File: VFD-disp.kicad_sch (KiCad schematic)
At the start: 96 parts, among them J1 USB_C_Receptacle_USB2.0_14P, J10 Conn_02x03_Odd_Even, J11 Conn_02x03_Odd_Even, J2 Conn_01x04_MountingPin, J3 Jack-DC, J8 Conn_02x03_Odd_Even, J9 Conn_02x03_Odd_Even, Q1 NMOS, Q3 NMOS, SW1 SW_SPST, U1 ESP32-C6-WROOM-1, U11 MAX811TEUS-T, U12 MCP4728, U2 FUSB302B01MPX, U3 LM1117DT-3.3, U4 MCP1416, U5 LM2576HVS-ADJ, U6 MAX1771xSA, U7 LM2576HVS-ADJ, U8 L7812, U9 FM24C64B, Y1 Crystal

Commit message: Make schematic ready for routing
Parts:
- removed F2: Fuse, Fuse:Fuse_0805_2012Metric, symbol Device:Fuse
- removed J10, J8: Conn_02x03_Odd_Even, Connector_PinSocket_2.54mm:PinSocket_2x03_P2.54mm_Horizontal, symbol Connector_Generic:Conn_02x03_Odd_Even
- removed J11, J9: Conn_02x03_Odd_Even, Connector_PinHeader_2.54mm:PinHeader_2x03_P2.54mm_Horizontal, symbol Connector_Generic:Conn_02x03_Odd_Even
- removed J2: Conn_01x04_MountingPin, Connector_JST:JST_SH_BM04B-SRSS-TB_1x04-1MP_P1.00mm_Vertical, symbol Connector_Generic_MountingPin:Conn_01x04_MountingPin
- removed R23: R, Resistor_SMD:R_0805_2012Metric, symbol Device:R
- added C19, C30, C31, C32, C33, C35: C, Capacitor_SMD:C_0805_2012Metric, symbol Device:C
- added C34: C_Polarized, Capacitor_Tantalum_SMD:CP_EIA-7343-31_Kemet-D, symbol Device:C_Polarized
- added J2, J5: Conn_02x04_Odd_Even, Connector_PinSocket_2.54mm:PinSocket_2x04_P2.54mm_Horizontal, symbol Connector_Generic:Conn_02x04_Odd_Even
- added J4, J6: Conn_02x04_Odd_Even, Connector_PinHeader_2.54mm:PinHeader_2x04_P2.54mm_Horizontal, symbol Connector_Generic:Conn_02x04_Odd_Even
- added R21: R, Resistor_SMD:R_0805_2012Metric, symbol Device:R
- added U10: TXS0104EPW, Package_SO:TSSOP-14_4.4x5mm_P0.65mm, symbol Logic_LevelTranslator:TXS0104EPW
- C18: footprint (none) -> Capacitor_SMD:C_0805_2012Metric
- R7: footprint (none) -> Resistor_SMD:R_0805_2012Metric
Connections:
- net +12V: no longer R3.1, U6.2 (V+)
- net +3.3V: now also R22.1, R3.1, C30.1, R21.1, U10.1 (V_{CCA})
- net +5V: now also C19.1, C33.1, C34.1, U10.14 (V_{CCB})
- net BLANKING: now also U10.11 (B3); no longer U1.17 (GPIO19)
- net CLOCK: now also U10.12 (B2); no longer U1.16 (GPIO18)
- net DATA_IN: now also U10.13 (B1); no longer U1.23 (GPIO15)
- net F_EN: now also R17.1, U1.19 (GPIO21); no longer R17.2
- net F_PWM: no longer U1.19 (GPIO21)
- net GND: now also R17.2, C19.2, C30.2, C31.2, C32.2, C33.2, C34.2, C35.2, J2.5 (Pin_5), J2.6 (Pin_6), J2.7 (Pin_7), J2.8 (Pin_8), J4.5 (Pin_5), J4.6 (Pin_6), J4.7 (Pin_7), J4.8 (Pin_8), J5.3 (Pin_3), J5.5 (Pin_5), J5.6 (Pin_6), J5.7 (Pin_7), J5.8 (Pin_8), J6.3 (Pin_3), J6.5 (Pin_5), J6.6 (Pin_6), J6.7 (Pin_7), J6.8 (Pin_8), U10.7 (GND), U10.8 (OE)
- net STROBE: now also U10.10 (B4); no longer U1.18 (GPIO20)
- net VBUS: now also U6.2 (V+), C35.1, J2.1 (Pin_1), J2.2 (Pin_2), J2.3 (Pin_3), J2.4 (Pin_4), J4.1 (Pin_1), J4.2 (Pin_2), J4.3 (Pin_3), J4.4 (Pin_4); no longer R17.1
- net TX2: now reaches U1.20 (GPIO22)
- net TX2: now also J6.4 (Pin_4)
- net RX2: now reaches U1.21 (GPIO23)
- net RX2: now also J6.2 (Pin_2)
- net at U1.26 (GPIO3/ADC1_CH3): now also R19.2, R20.1
- net at U1.27 (GPIO2/ADC1_CH2): now also C18.1, R15.2, R18.1
- net at J1.B5 (CC2), U2.1 (CC2), U2.14 (CC2): now also C32.1
- net at J1.A5 (CC1), U2.10 (CC1), U2.11 (CC1): now also C31.1
- net DATA_OUT: no longer names the net of HV5812WG2.2 (DATAOUT)
- net HV_EN renamed /HV_EN
- net RX renamed RX1
- net RX1: now also J5.4 (Pin_4)
- net TX renamed FORWARD_DETECT
- net FORWARD_DETECT: now also U1.5 (MTDI/GPIO5/ADC1_CH5), J6.1 (Pin_1); no longer U1.25 (U0TXD/GPIO16)
- new net: U1.23 (GPIO15), U10.2 (A1)
- new net: U1.16 (GPIO18), U10.3 (A2)
- new net: U1.17 (GPIO19), U10.4 (A3)
- new net: U1.18 (GPIO20), U10.5 (A4)
- new net BACKWARD_DETECT: J5.1 (Pin_1), R21.2, U1.4 (MTMS/GPIO4/ADC1_CH4)
- new net TX1: J5.2 (Pin_2), U1.25 (U0TXD/GPIO16)
- no-connect marks 15 -> 16
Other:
- moved on the sheet: C15, C16, C17, C18, C27, C29, R13, R14, R15, R17, R18, R19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

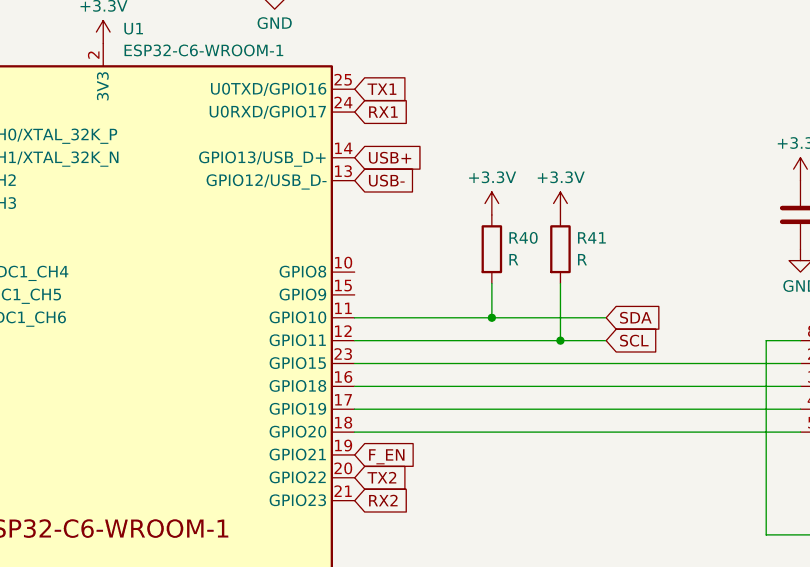
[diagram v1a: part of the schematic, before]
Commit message: WIP płytka
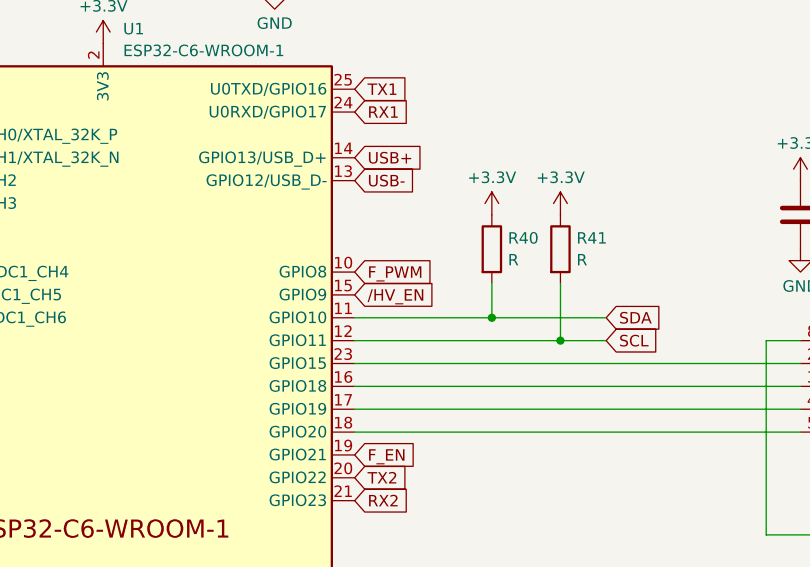
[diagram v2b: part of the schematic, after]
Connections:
- net F_PWM: now also U1.10 (GPIO8)
- net /HV_EN: now also U1.15 (GPIO9)
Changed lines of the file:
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@@
+		)
+	)
+	(global_label "F_PWM"
+		(shape input)
+		(at 224.79 102.87 0)
+		(fields_autoplaced yes)
+		(effects
+			(font
+				(size 1.27 1.27)
+			)
+			(justify left)
+		)
+		(property "Intersheetrefs" "${INTERSHEET_REFS}"
+			(at 234.0042 102.87 0)
+			(effects
+				(font
+					(size 1.27 1.27)
+				)
+				(justify left)
+				(hide yes)
+			)
 		)
 	)
@@
 				(hide yes)
 			)
+		)
+	)
+	(global_label "{slash}HV_EN"
+		(shape input)
+		(at 224.79 105.41 0)
+		(fields_autoplaced yes)
+		(effects
+			(font
+				(size 1.27 1.27)
+			)
+			(justify left)
+		)
+		(property "Intersheetrefs" "${INTERSHEET_REFS}"
+			(at 234.9719 105.41 0)
+			(effects
+				(font
+					(size 1.27 1.27)
+				)
+				(justify left)
+				(hide yes)
+			)

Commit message: WIP płytka
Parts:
- removed C10, C9: C_Polarized, Capacitor_SMD:CP_Elec_5x4.5, symbol Device:C_Polarized
- removed C14, C8: C, Capacitor_SMD:C_0805_2012Metric, symbol Device:C
- removed U8: L7812, Package_TO_SOT_SMD:TO-252-2, symbol Regulator_Linear:L7812
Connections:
- net USB+ is gone; now on net USB_D+: U1.14 (GPIO13/USB_D+)
- net USB- is gone; now on net USB_D-: U1.13 (GPIO12/USB_D-)
- net BACKWARD_DETECT: now also U1.5 (MTDI/GPIO5/ADC1_CH5); no longer U1.4 (MTMS/GPIO4/ADC1_CH4)
- net FORWARD_DETECT: now also J6.3 (Pin_3), U1.4 (MTMS/GPIO4/ADC1_CH4); no longer J6.1 (Pin_1), U1.5 (MTDI/GPIO5/ADC1_CH5)
- net GND: now also J5.2 (Pin_2), J5.4 (Pin_4), J6.1 (Pin_1), J6.2 (Pin_2), J6.4 (Pin_4); no longer J5.5 (Pin_5), J5.7 (Pin_7), J6.3 (Pin_3), J6.5 (Pin_5), J6.7 (Pin_7)
- net RX1: now also J6.5 (Pin_5); no longer J5.4 (Pin_4)
- net RX2: now also J5.7 (Pin_7); no longer J6.2 (Pin_2)
- net TX1: now also J6.7 (Pin_7); no longer J5.2 (Pin_2)
- net TX2: now also J5.5 (Pin_5); no longer J6.4 (Pin_4)
- net at R4.1, U6.8 (CS): now also Q1.1 (D); no longer Q1.3 (S)
- net at D1.2 (A), L1.2: now also Q1.3 (S); no longer Q1.1 (D)
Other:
- moved on the sheet: R22

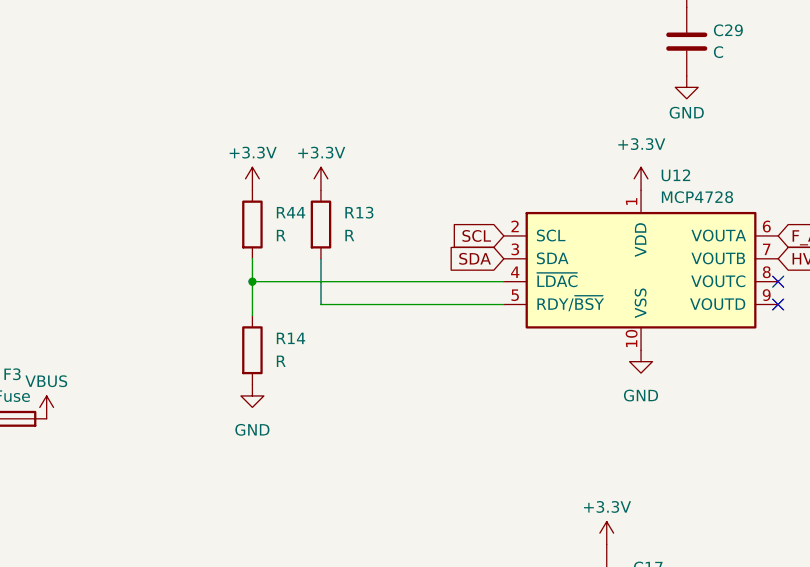
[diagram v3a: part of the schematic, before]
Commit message: WIP płytka
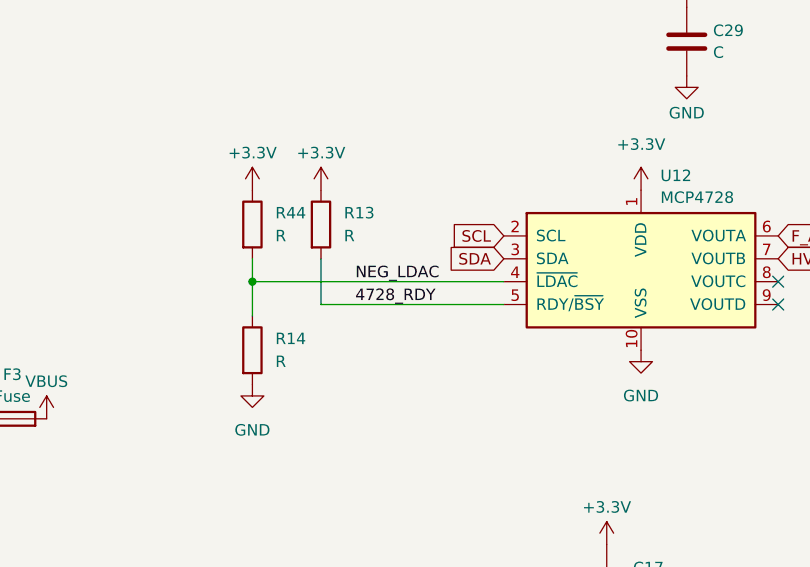
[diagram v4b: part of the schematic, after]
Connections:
- net 4728_RDY: now reaches R13.2, U12.5 (RDY/~{BSY})
- net NEG_LDAC: now reaches R14.1, R44.2, U12.4 (~{LDAC})
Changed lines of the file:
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@@
+		)
+	)
+	(label "4728_RDY"
+		(at 87.63 304.8 0)
+		(effects
+			(font
+				(size 1.27 1.27)
+			)
+			(justify left bottom)
 		)
 	)
@@
 		(effects
 			(font
+				(size 1.27 1.27)
+			)
+			(justify left bottom)
+		)
+	)
+	(label "NEG_LDAC"
+		(at 87.63 302.26 0)
+		(effects
+			(font

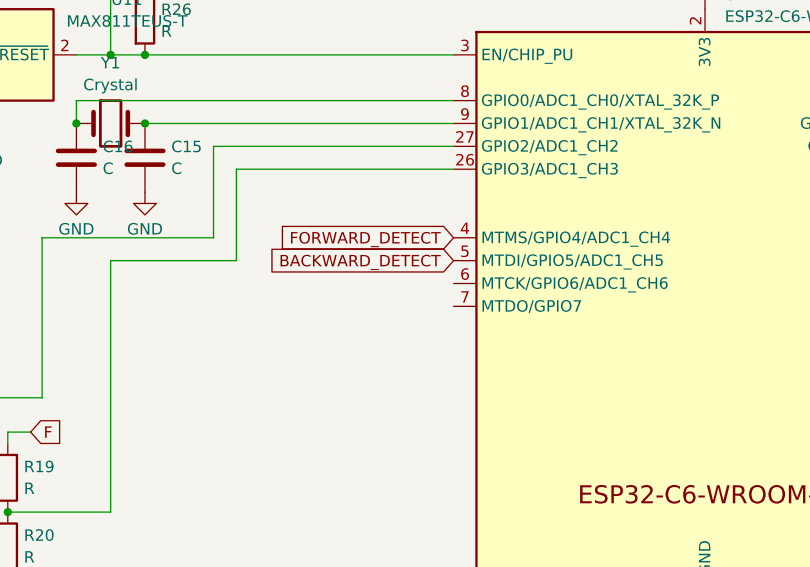
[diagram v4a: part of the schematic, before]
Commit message: WIP płytka
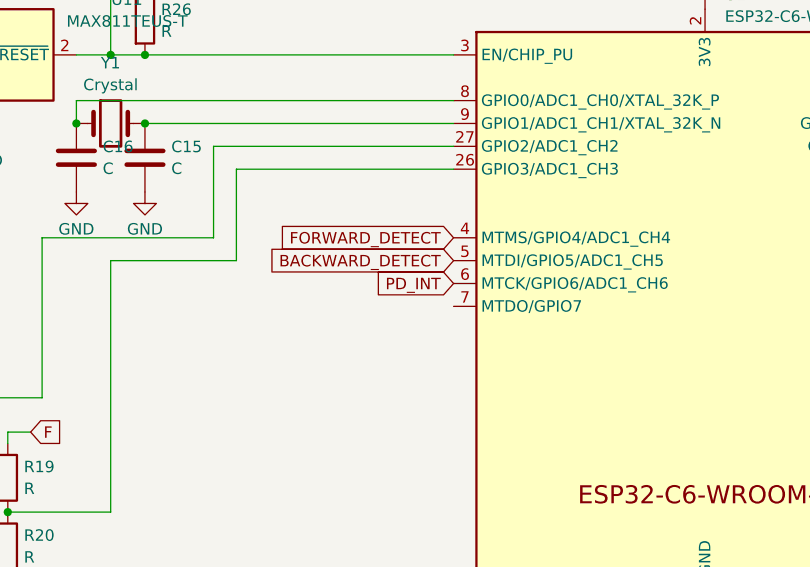
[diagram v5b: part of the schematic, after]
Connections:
- net PD_INT: now also U1.6 (MTCK/GPIO6/ADC1_CH6)
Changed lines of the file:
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@@
+		)
+	)
+	(global_label "PD_INT"
+		(shape input)
+		(at 168.91 107.95 180)
+		(fields_autoplaced yes)
+		(effects
+			(font
+				(size 1.27 1.27)
+			)
+			(justify right)
+		)
+		(property "Intersheetrefs" "${INTERSHEET_REFS}"
+			(at 159.5143 107.95 0)
+			(effects
+				(font
+					(size 1.27 1.27)
+				)
+				(justify right)
+				(hide yes)
+			)
 		)
 	)

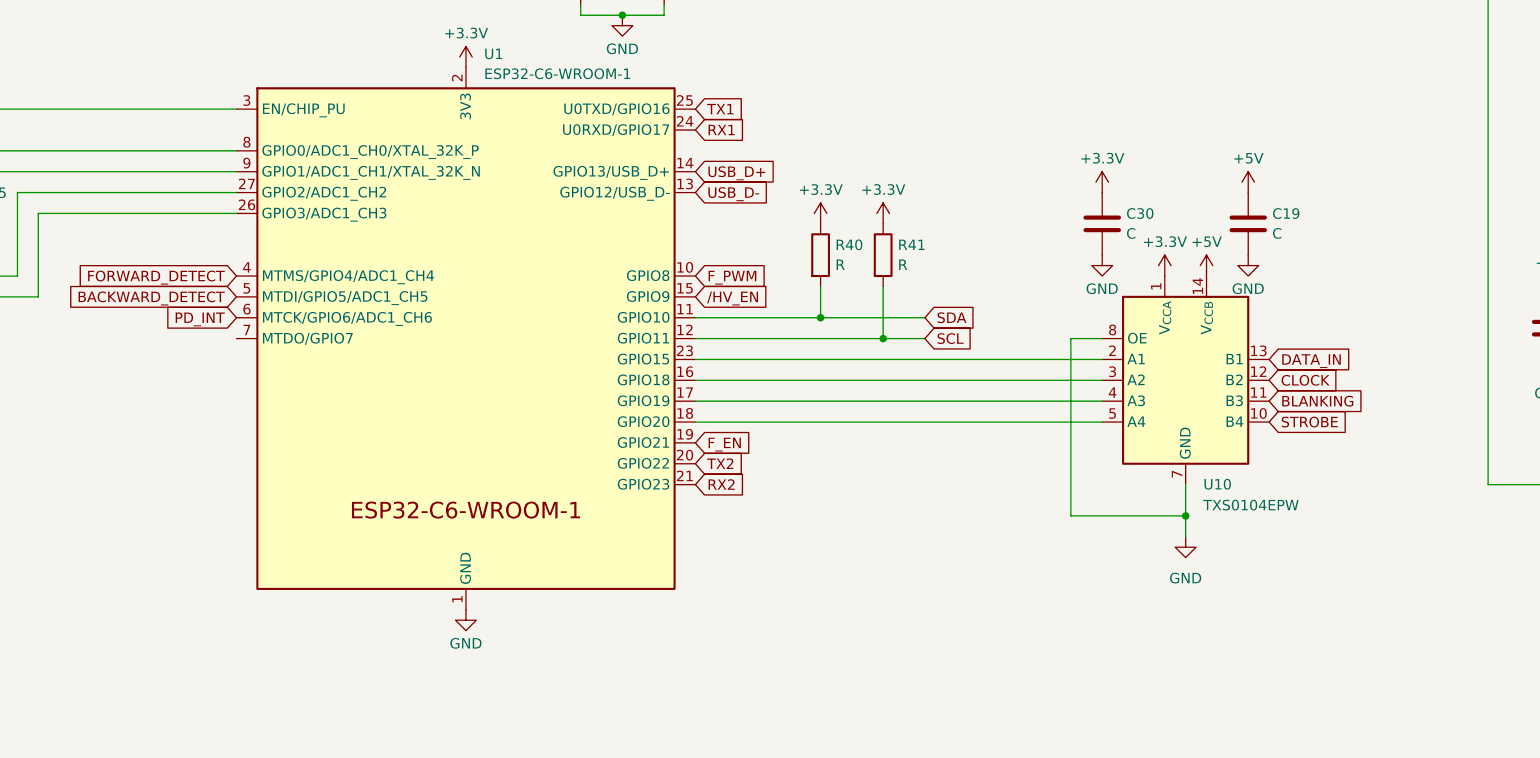
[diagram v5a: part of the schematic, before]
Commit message: WIP all components placed
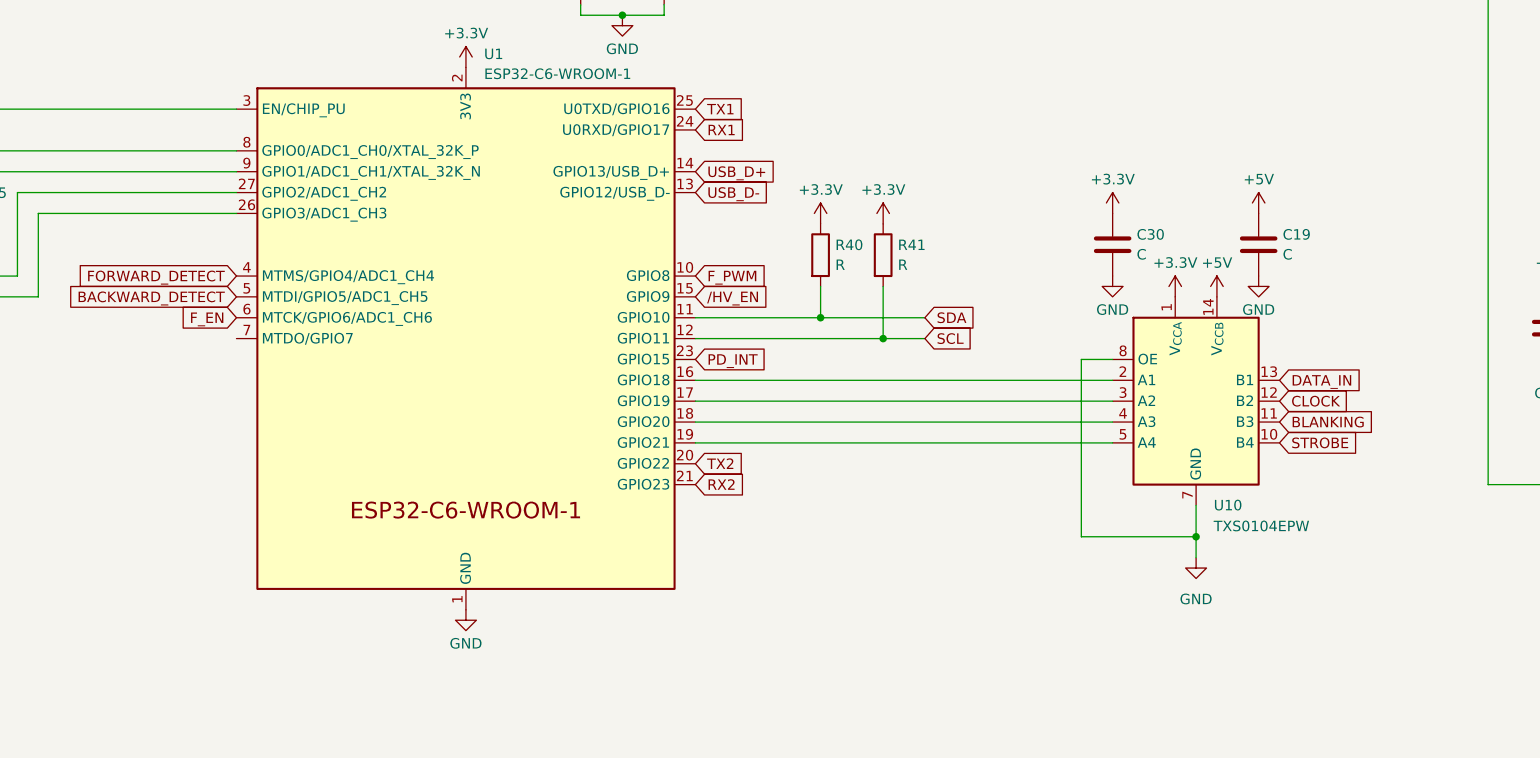
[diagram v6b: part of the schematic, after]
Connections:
- net F_EN: now also U1.6 (MTCK/GPIO6/ADC1_CH6); no longer U1.19 (GPIO21)
- net PD_INT: now also U1.23 (GPIO15); no longer U1.6 (MTCK/GPIO6/ADC1_CH6)
- net at U10.2 (A1): now also U1.16 (GPIO18); no longer U1.23 (GPIO15)
- net at U10.3 (A2): now also U1.17 (GPIO19); no longer U1.16 (GPIO18)
- net at U10.4 (A3): now also U1.18 (GPIO20); no longer U1.17 (GPIO19)
- net at U10.5 (A4): now also U1.19 (GPIO21); no longer U1.18 (GPIO20)
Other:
- moved on the sheet: C19, C30, U10

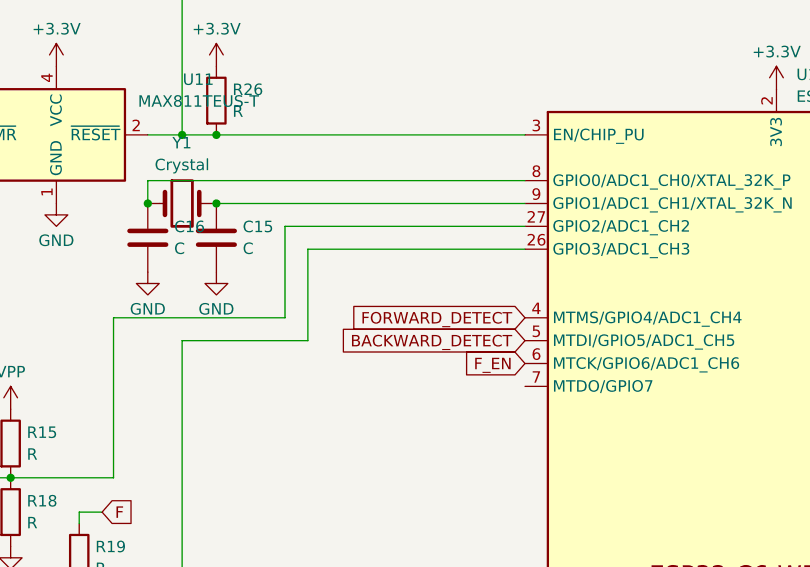
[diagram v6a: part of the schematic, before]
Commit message: WIP connecting...
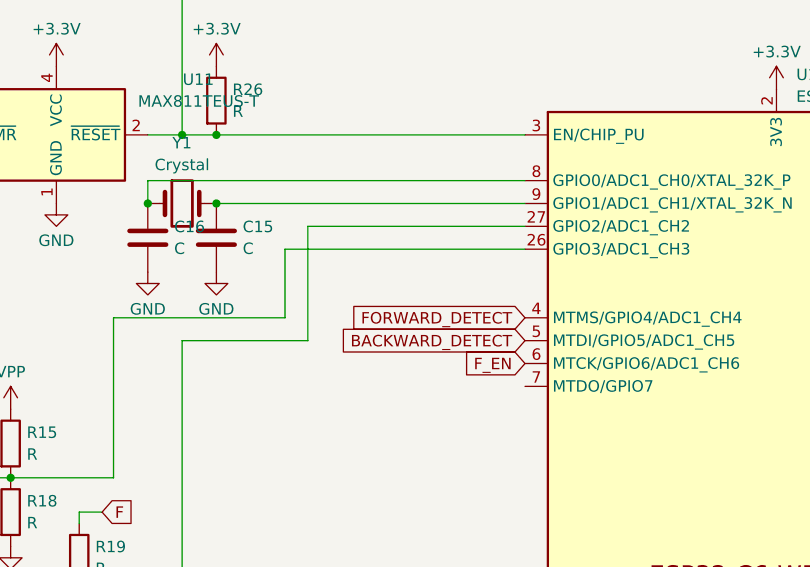
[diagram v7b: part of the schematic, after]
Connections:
- net at R19.2, R20.1: now also U1.27 (GPIO2/ADC1_CH2); no longer U1.26 (GPIO3/ADC1_CH3)
- net at C18.1, R15.2, R18.1: now also U1.26 (GPIO3/ADC1_CH3); no longer U1.27 (GPIO2/ADC1_CH2)
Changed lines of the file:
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@@
+	(wire
+		(pts
+			(xy 142.24 102.87) (xy 142.24 95.25)
+		)
+		(stroke
+			(width 0)
+			(type default)
+		)
+	)
 	(wire
 		(pts
@@
 	(wire
 		(pts
-			(xy 142.24 92.71) (xy 168.91 92.71)
-		)
-		(stroke
-			(width 0)
-			(type default)
-		)
-	)
-	(wire
-		(pts
 			(xy 365.76 140.97) (xy 384.81 140.97)
 		)
@@
 	(wire
 		(pts
+			(xy 142.24 95.25) (xy 168.91 95.25)
+		)
+		(stroke
+			(width 0)
+			(type default)
+		)
+	)
+	(wire
+		(pts
 			(xy 302.26 265.43) (xy 302.26 267.97)
 		)
@@
 	(wire
 		(pts
-			(xy 144.78 105.41) (xy 144.78 95.25)
+			(xy 144.78 92.71) (xy 144.78 105.41)
 		)
 		(stroke
@@
 	(wire
 		(pts
-			(xy 142.24 102.87) (xy 142.24 92.71)
-		)
-		(stroke
-			(width 0)
-			(type default)
-		)
-	)
-	(wire
-		(pts
 			(xy 273.05 234.95) (xy 275.59 234.95)
 		)
@@
 	(wire
 		(pts
+			(xy 144.78 92.71) (xy 168.91 92.71)
+		)
+		(stroke
+			(width 0)
+			(type default)
+		)
+	)
+	(wire
+		(pts
 			(xy 257.81 260.35) (xy 290.83 260.35)
 		)
@@
 		)
 		(stroke
-			(width 0)
-			(type default)
-		)
-	)
-	(wire
-		(pts
-			(xy 144.78 95.25) (xy 168.91 95.25)
-		)
-		(stroke
